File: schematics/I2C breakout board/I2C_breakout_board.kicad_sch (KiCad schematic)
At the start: 7 parts, among them J1 Conn_01x07_Pin, J2 Conn_01x07_Pin, U1 ENS210-LQFM, U2 OPT4001DTSR

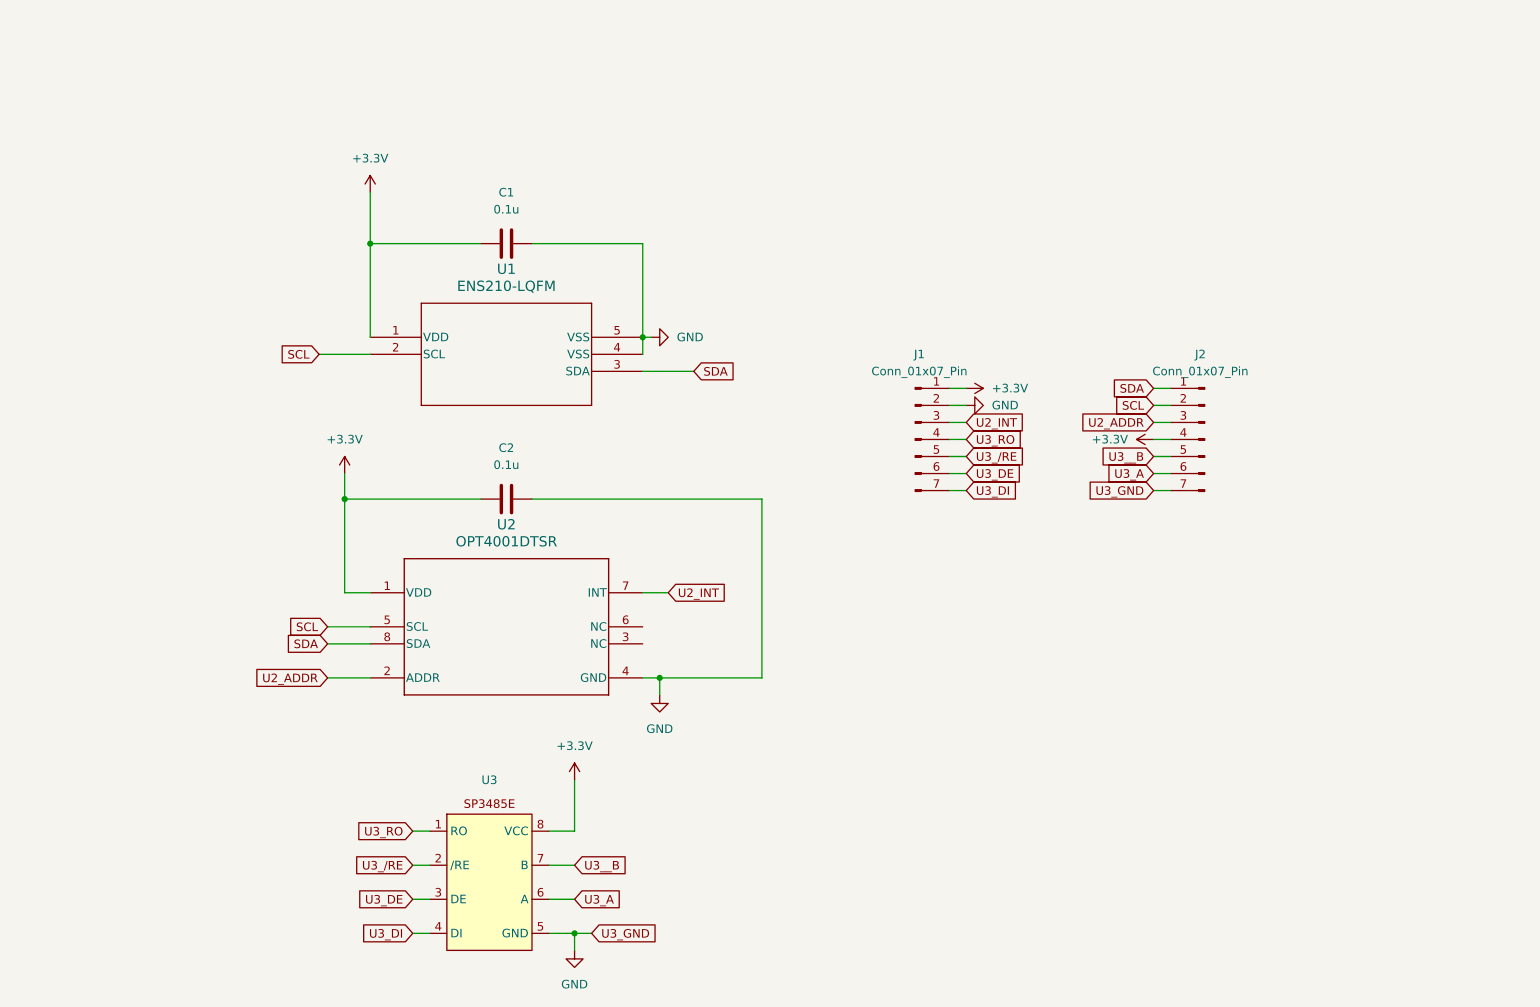
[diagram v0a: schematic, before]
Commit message: final version of air sensors breakout board
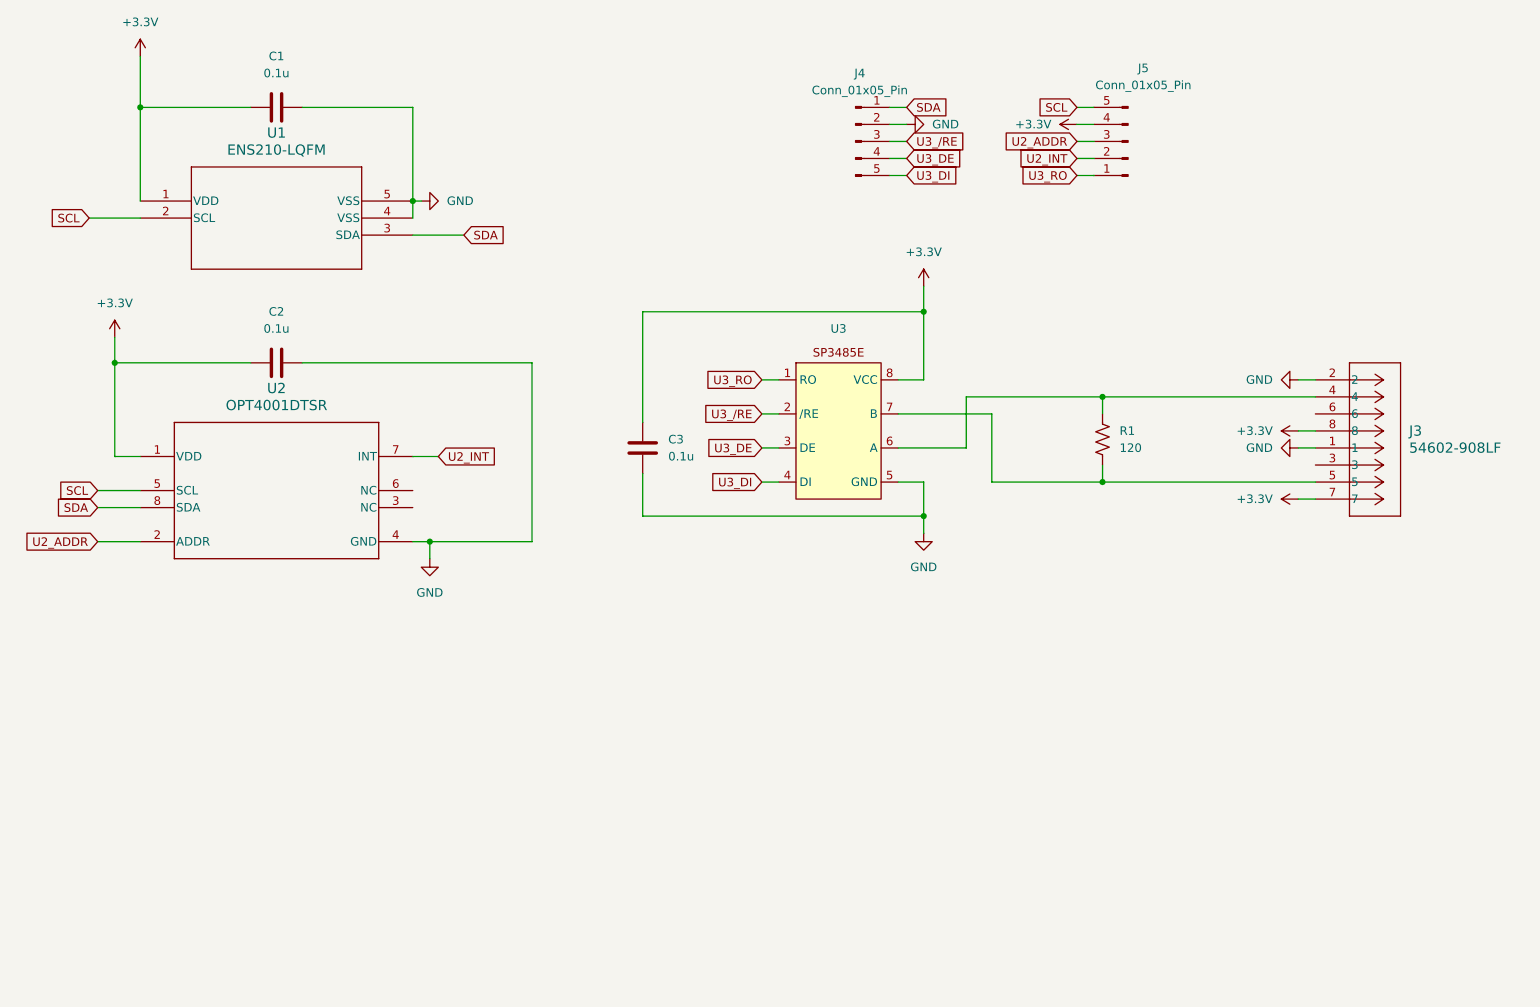
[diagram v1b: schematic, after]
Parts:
- removed J1, J2: Conn_01x07_Pin, Connector_PinHeader_2.54mm:PinHeader_1x07_P2.54mm_Vertical, symbol Connector:Conn_01x07_Pin
- added C3: 0.1u, Capacitor_SMD:C_0805_2012Metric_Pad1.18x1.45mm_HandSolder, symbol Device:C
- added J3: 54602-908LF, 54602_908LF_footprints:CONN8_2-908LF_AMP, symbol 2026-10-21_23-02-14:54602-908LF
- added J4, J5: Conn_01x05_Pin, Connector_PinHeader_2.54mm:PinHeader_1x05_P2.54mm_Vertical, symbol Connector:Conn_01x05_Pin
- added R1: 120, Resistor_SMD:R_0805_2012Metric_Pad1.20x1.40mm_HandSolder, symbol Device:R_US
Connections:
- net +3.3V: now also C3.2, J3.7, J3.8, J5.4 (Pin_4)
- net GND: now also C3.1, J3.1, J3.2, J4.2 (Pin_2)
- net SCL: now also J5.5 (Pin_5)
- net SDA: now also J4.1 (Pin_1)
- net U2_ADDR: now also J5.3 (Pin_3)
- net U2_INT: now also J5.2 (Pin_2)
- net U3_DE: now also J4.4 (Pin_4)
- net U3_DI: now also J4.5 (Pin_5)
- net U3_RO: now also J5.1 (Pin_1)
- net U3_/RE: now also J4.3 (Pin_3)
- net U3_A: no longer names the net of U3.6 (A)
- net U3_A: now also J3.4, R1.1
- net U3__B: no longer names the net of U3.7 (B)
- net U3__B: now also J3.5, R1.2
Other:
- moved on the sheet: C1, C2, U1, U2, U3
